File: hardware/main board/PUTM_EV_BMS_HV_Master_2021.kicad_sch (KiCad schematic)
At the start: 19 parts, among them U2 STM32G484RETx, Y1 20MHz, Y2 32.768kHz

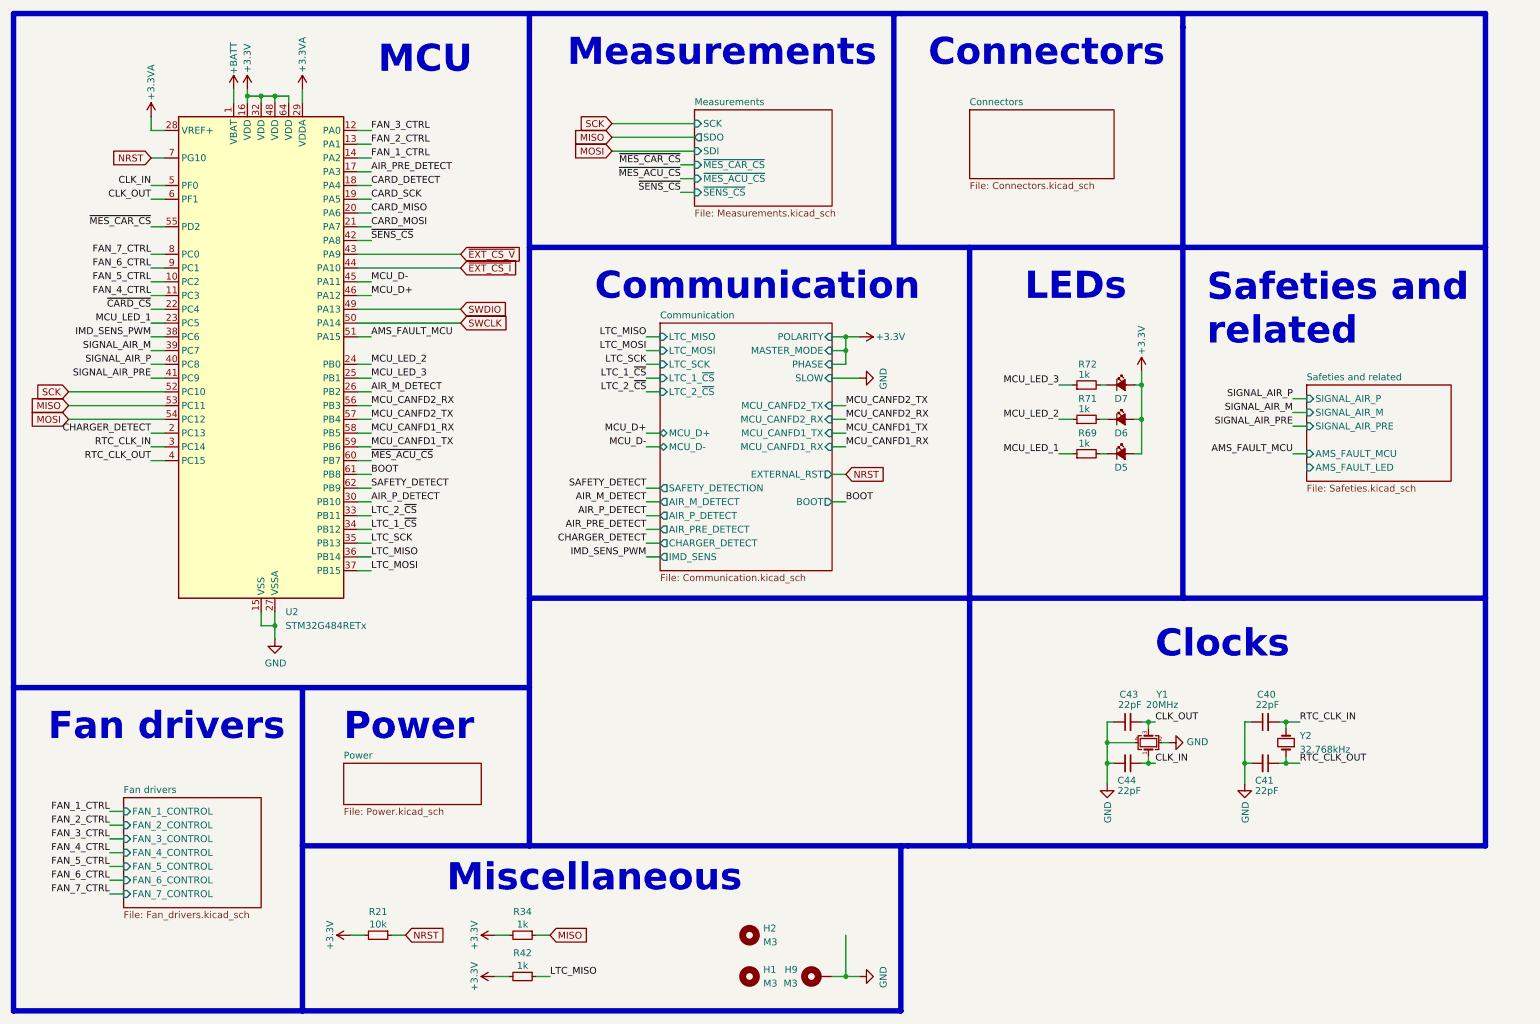
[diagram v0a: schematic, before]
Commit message: repairing demaged branch~
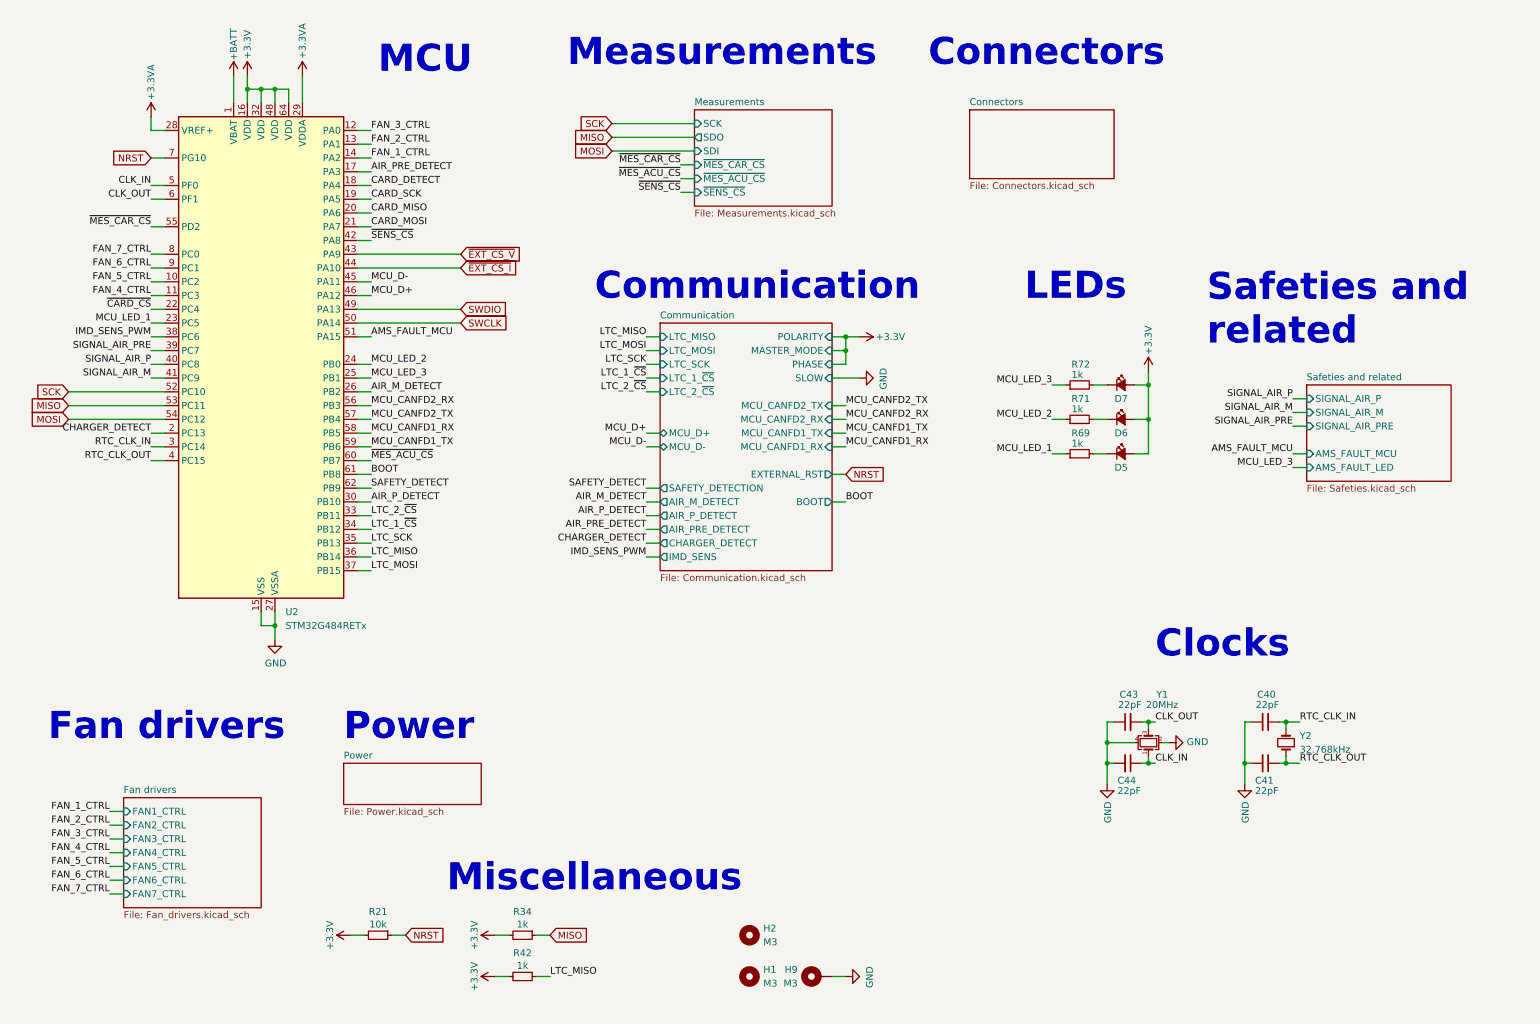
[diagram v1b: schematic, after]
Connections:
- net SIGNAL_AIR_M: now also U2.41 (PC9); no longer U2.39 (PC7)
- net SIGNAL_AIR_PRE: now also U2.39 (PC7); no longer U2.41 (PC9)
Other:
- sheet Fan drivers ports: added FAN1_CTRL, FAN2_CTRL, FAN3_CTRL, FAN4_CTRL, FAN5_CTRL, FAN6_CTRL, FAN7_CTRL; removed FAN_1_CONTROL, FAN_2_CONTROL, FAN_3_CONTROL, FAN_4_CONTROL, FAN_5_CONTROL, FAN_6_CONTROL, FAN_7_CONTROL
- moved on the sheet: R69, R71, R72
